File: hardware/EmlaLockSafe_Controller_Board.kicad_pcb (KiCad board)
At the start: 4 copper layers, 11 parts, among them Q1 IRLML6244

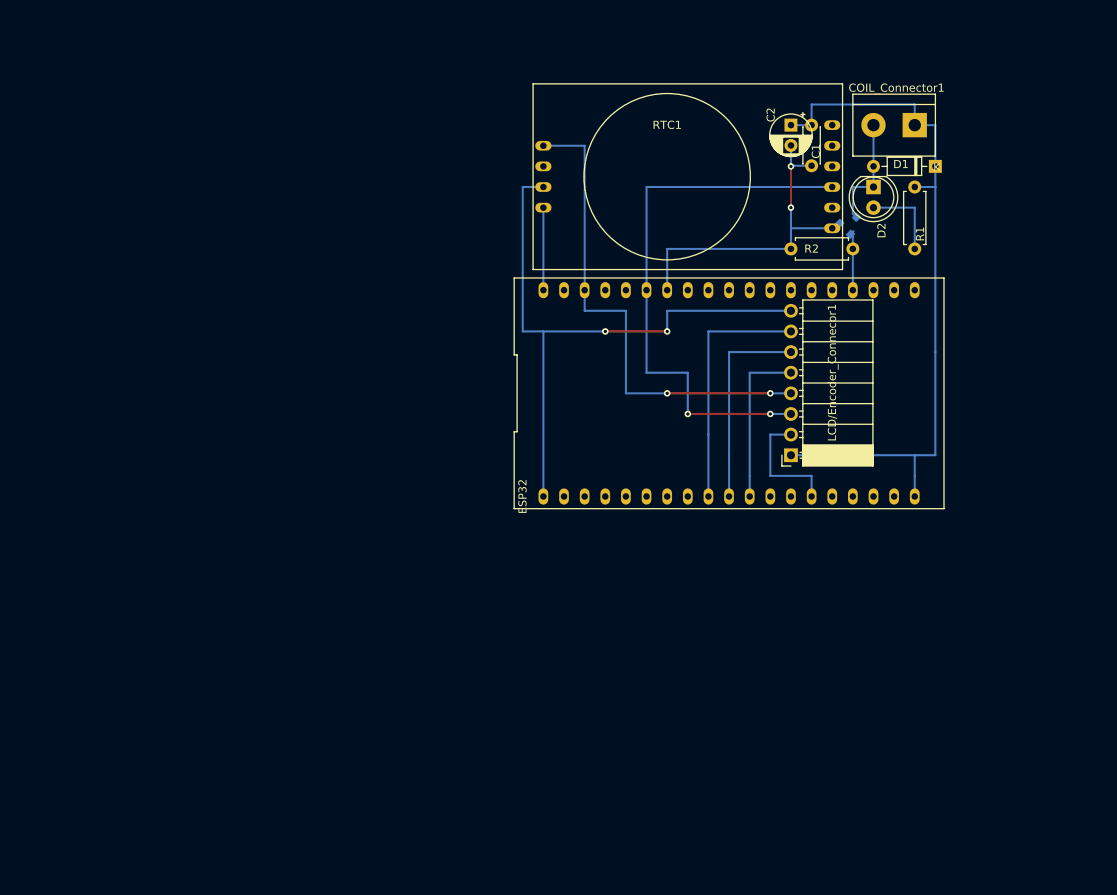
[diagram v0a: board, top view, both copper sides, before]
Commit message: Updated schematics
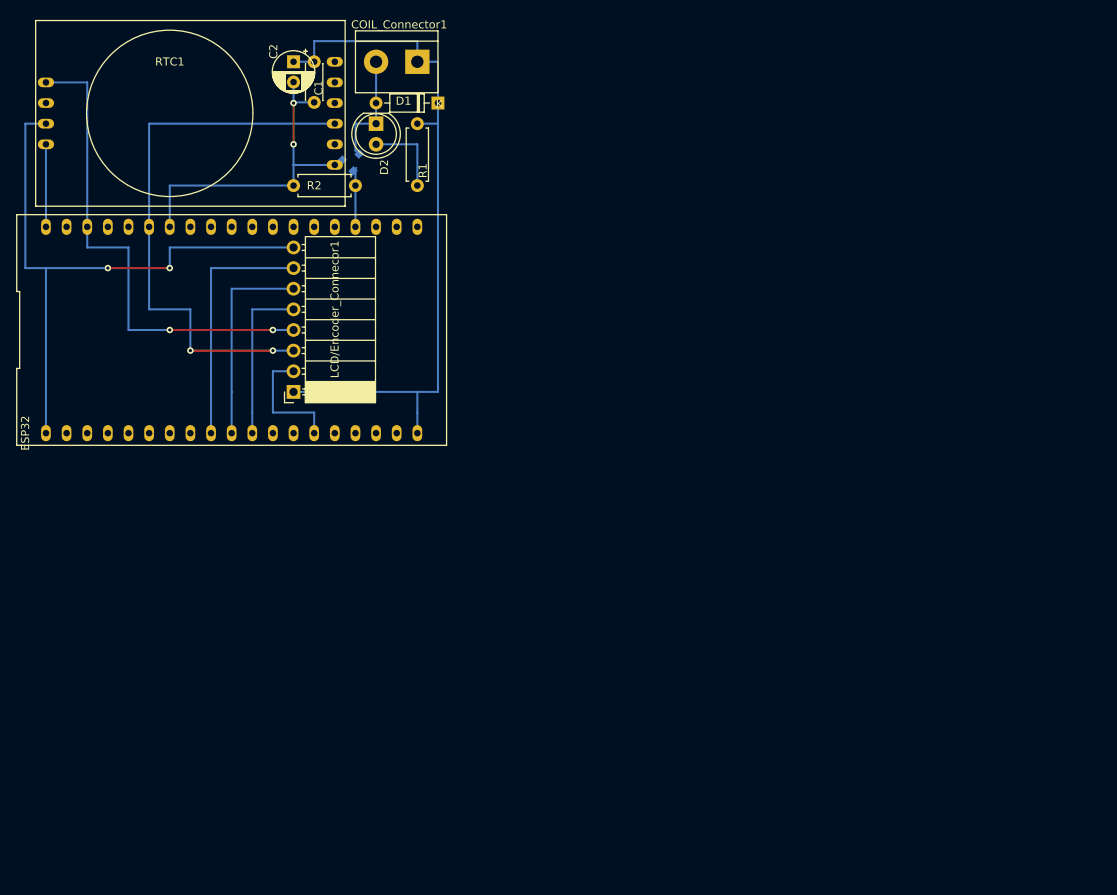
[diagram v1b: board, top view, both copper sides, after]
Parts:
- moved COIL_Connector1 61.7 mm to (88.6, 32.8)
- moved R1 61.7 mm to (88.6, 48.1)
- moved C1 61.7 mm to (75.9, 32.8)
- moved C2 61.7 mm to (73.4, 32.8)
- moved D1 61.7 mm to (91.2, 37.9)
- moved R2 61.7 mm to (73.4, 48.1)
- moved RTC1 61.7 mm to (60.7, 39.2)
- moved D2 61.7 mm to (83.5, 40.5)
- moved ESP32 61.7 mm to (65.8, 65.9)
- moved LCD/Encoder_Connecor1 61.7 mm to (73.4, 73.5)
- moved Q1 61.7 mm to (80.7, 44.9)

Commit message: Updated to V2
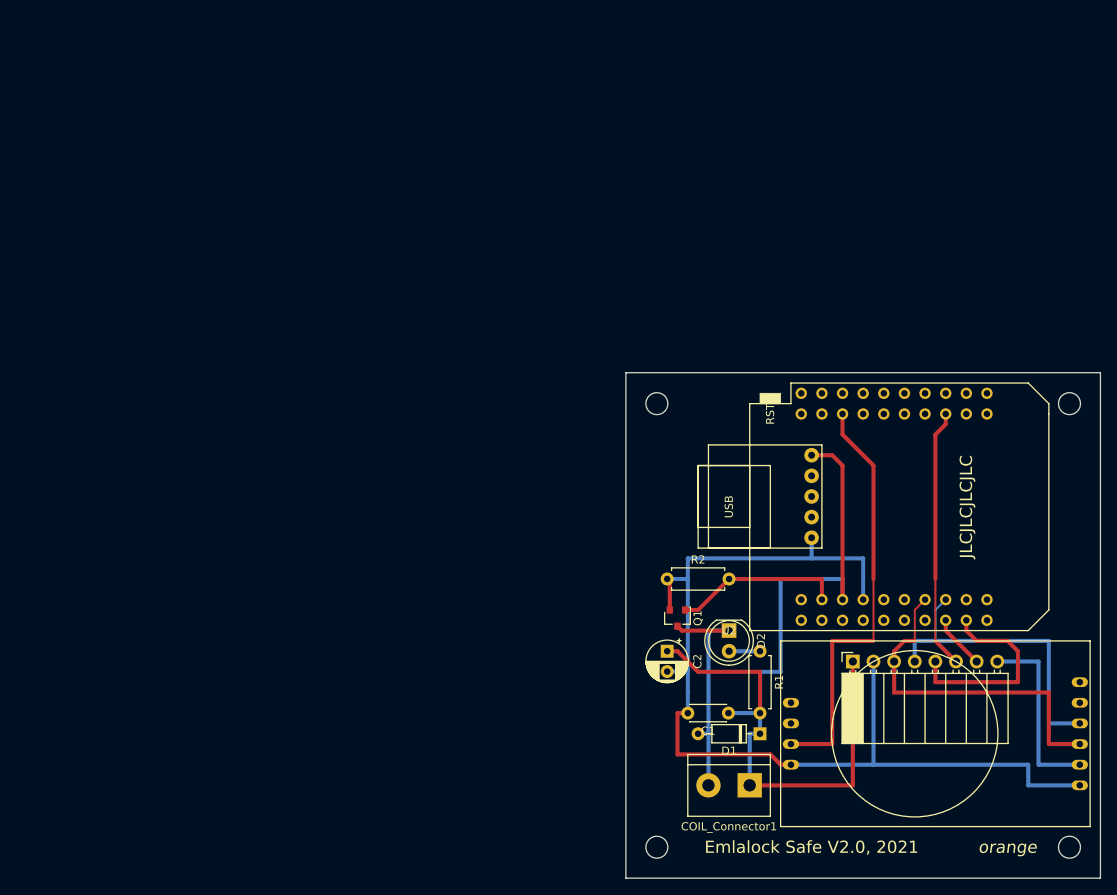
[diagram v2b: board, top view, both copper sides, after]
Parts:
- removed ESP32: ESP32_NodeMCU_Module_AzDelivery, ESP32_NodeMCU_Module_AzDelivery:ESP32_NodeMCU_Module_AzDelivery
- added REF**: MountingHole_2.7mm_M2.5, MountingHole:MountingHole_2.7mm_M2.5, F.Cu at (168.9, 74.9)
- added REF**: MountingHole_2.7mm_M2.5, MountingHole:MountingHole_2.7mm_M2.5, F.Cu at (168.9, 129.5)
- added REF**: MountingHole_2.7mm_M2.5, MountingHole:MountingHole_2.7mm_M2.5, F.Cu at (118.1, 129.5)
- added REF**: MountingHole_2.7mm_M2.5, MountingHole:MountingHole_2.7mm_M2.5, F.Cu at (118.1, 74.9)
- added U1: mini_esp32, ESP32_mini_KiCad_Library:ESP32_mini, F.Cu at (147.3, 87.6)
- added U2: MicroUSBBreakout, MicroUSBBreakout:MicroUSBBreakout, F.Cu at (130.8, 86.4)
- Q1: moved to F.Cu
- moved RTC1 119.4 mm to (152.4, 115.6)
- moved COIL_Connector1 98.0 mm to (129.5, 121.9)
- moved C1 95.0 mm to (126.9, 113.0), turned to 180 degrees
- moved D1 87.2 mm to (130.8, 115.6)
- moved C2 85.9 mm to (119.4, 105.4)
- moved LCD/Encoder_Connecor1 76.4 mm to (142.2, 106.7), turned to 90 degrees
- moved D2 76.0 mm to (127.0, 102.9)
- moved R1 71.2 mm to (130.8, 105.4), turned to 270 degrees
- moved Q1 69.1 mm to (120.7, 101.3), turned to 270 degrees
- moved R2 66.8 mm to (119.4, 96.5)
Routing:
- net SDA: track 105.4 -> 43.0 mm, vias 2 -> 0
- net SCL: track 98.9 -> 38.6 mm, vias 2 -> 0
- net +3V3: track 112.8 -> 75.2 mm, vias 2 -> 0
- net ENC_SW: track 30.5 -> 6.66 mm
- net +5V: track 88.9 -> 109.6 mm
- net Net-(COIL_Connector1-Pad2): track 14.1 -> 30.2 mm
- net COIL: track 7.55 -> 20.9 mm
- net GND: track 119.5 -> 128.9 mm, vias 2 -> 0
- net ENC_DT: track 25.4 -> 32.1 mm
- net Net-(D2-Pad2): track 10.2 -> 3.81 mm
- net ENC_CLK: track 20.3 -> 25.2 mm
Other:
- board outline added: 58.4 x 62.2 mm
- copper layers 4 -> 2
- rule pad_to_mask_clearance: 0.051 -> 0
- board text added: "Emlalock Safe V2.0, 2021"
- board text added: "JLCJLCJLCJLC"
- board text added: "orange"
